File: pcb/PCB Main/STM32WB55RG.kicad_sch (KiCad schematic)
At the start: 26 parts, among them CN1 Conn_ARM_JTAG_SWD_10, SW1 SW_Push, U1 STM32WB55RGVx, Y1 32MHz, Y2 32.768kHz

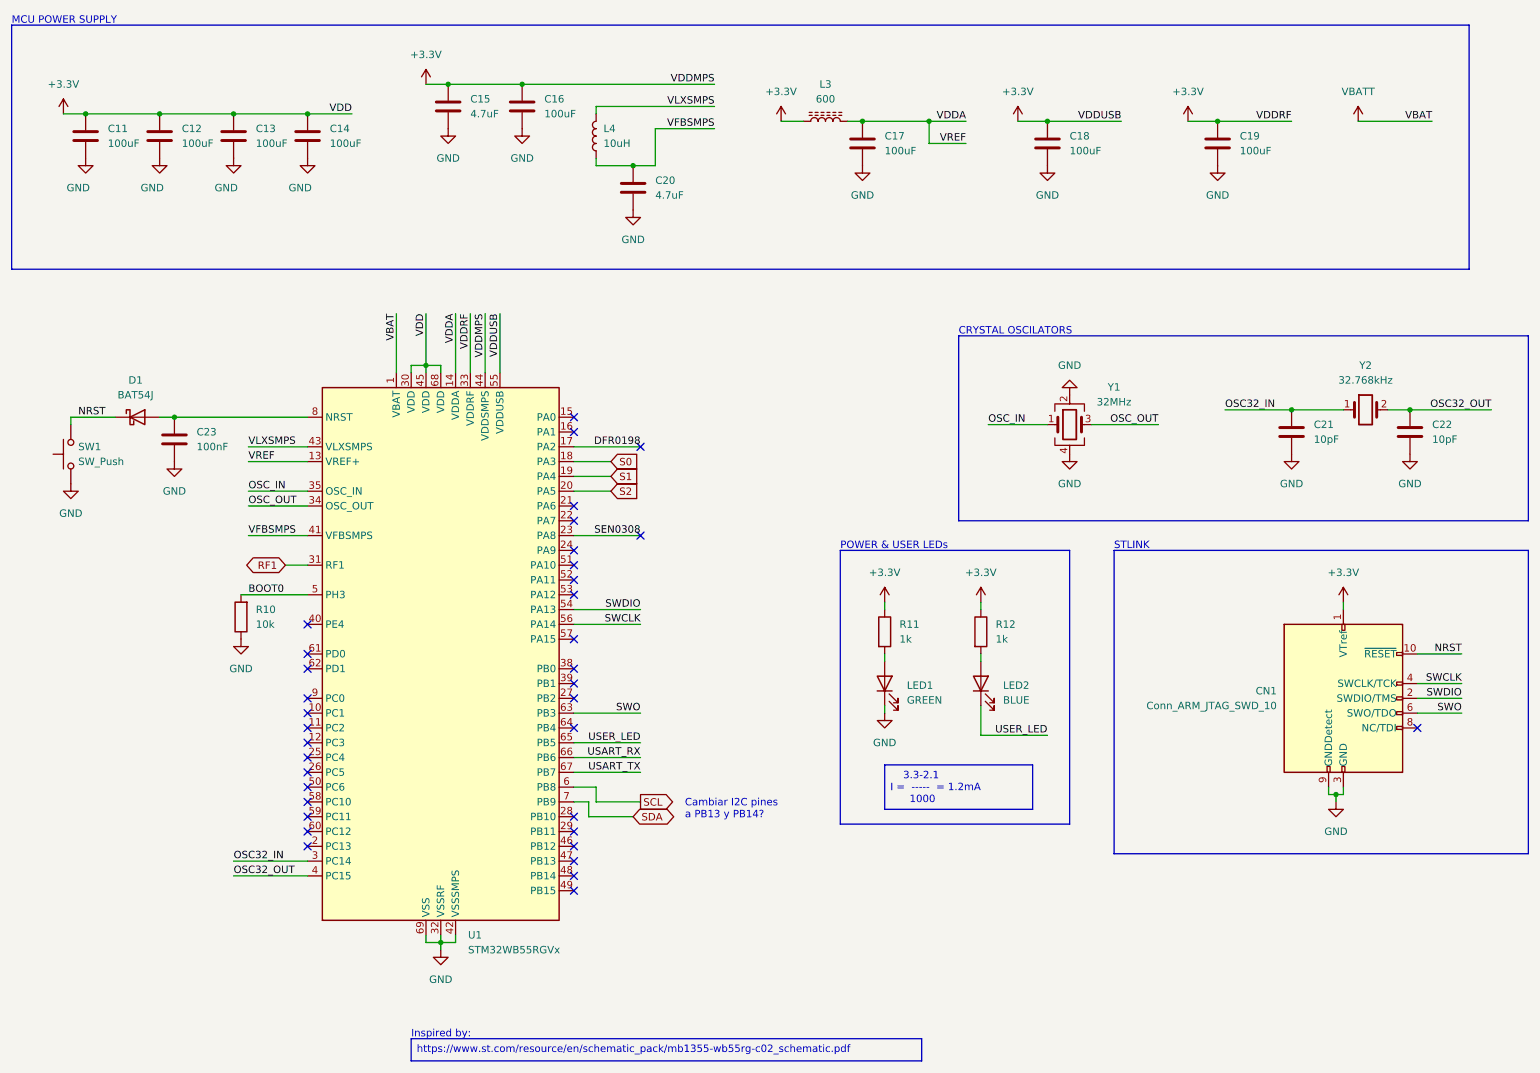
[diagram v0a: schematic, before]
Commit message: PCB casi lista
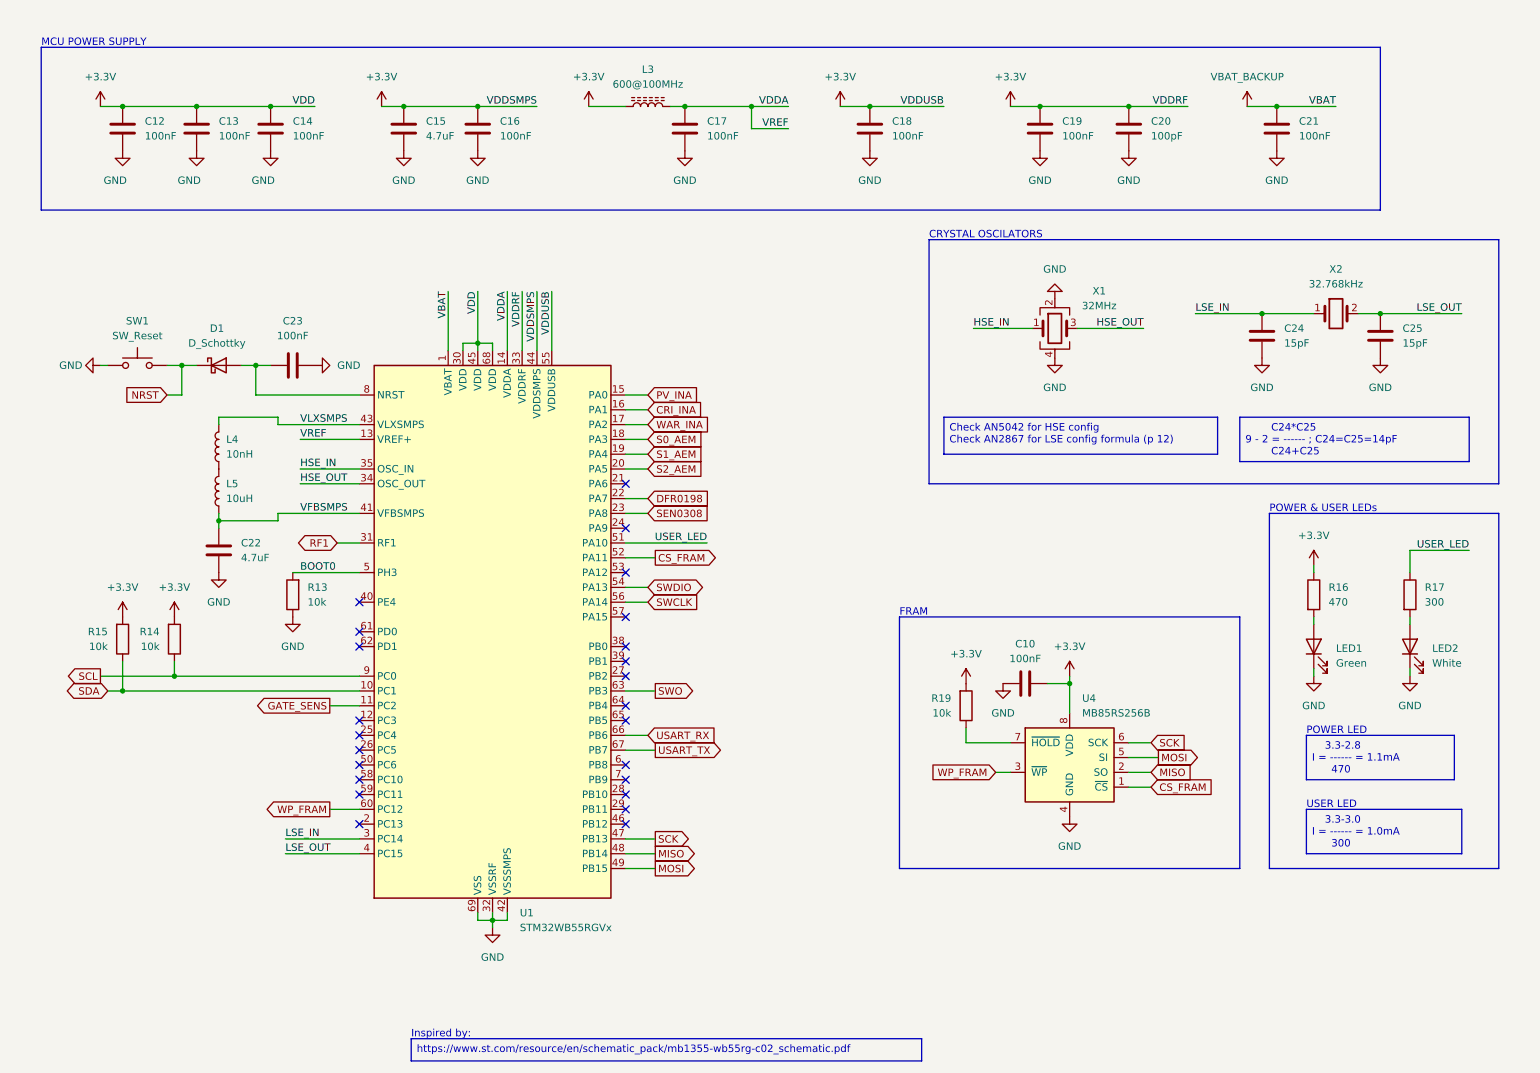
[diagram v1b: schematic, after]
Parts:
- removed C11: 100uF, symbol Device:C
- removed CN1: Conn_ARM_JTAG_SWD_10, Connector_PinHeader_1.27mm:PinHeader_2x05_P1.27mm_Vertical, symbol Connector:Conn_ARM_JTAG_SWD_10
- removed D1: BAT54J, Diode_SMD:D_SOD-323F, symbol Diode:BAT54J
- added C10, C21: 100nF, Capacitor_SMD:C_0402_1005Metric, symbol Device:C
- added C20: 100pF, Capacitor_SMD:C_0402_1005Metric, symbol Device:C
- added D1: D_Schottky, Diode_SMD:D_SOD-323, symbol Device:D_Schottky
- added L4: 10nH, Inductor_SMD:L_0402_1005Metric, symbol Device:L
- added R14, R15, R19: 10k, Resistor_SMD:R_0402_1005Metric, symbol Device:R
- added U4: MB85RS256B, Package_SO:SOIC-8_3.9x4.9mm_P1.27mm, symbol Memory_NVRAM:MB85RS256B
- C12, C13, C14, C16, C17, C18, C19: value 100uF -> 100nF; footprint (none) -> Capacitor_SMD:C_0402_1005Metric; Component (none) -> CL05B104KO5NNNC; Manufacturer (none) -> Samsung; Package (none) -> 0402; Supplier (none) -> JLCPCB; Supplier Part # (none) -> C1525; Supplier Part Type (none) -> Basic
- C15: footprint (none) -> Capacitor_SMD:C_0402_1005Metric; Component (none) -> CL05A475MP5NRNC; Manufacturer (none) -> Samsung; Package (none) -> 0402; Supplier (none) -> JLCPCB; Supplier Part # (none) -> C23733; Supplier Part Type (none) -> Basic
- C22: renamed from C20; footprint (none) -> Capacitor_SMD:C_0402_1005Metric; Component (none) -> CL05A475MP5NRNC; Manufacturer (none) -> Samsung; Package (none) -> 0402; Supplier (none) -> JLCPCB; Supplier Part # (none) -> C23733; Supplier Part Type (none) -> Basic
- C23: footprint (none) -> Capacitor_SMD:C_0402_1005Metric; Component (none) -> CL05B104KO5NNNC; Manufacturer (none) -> Samsung; Package (none) -> 0402; Supplier (none) -> JLCPCB; Supplier Part # (none) -> C1525; Supplier Part Type (none) -> Basic
- C24: renamed from C21; value 10pF -> 15pF; footprint (none) -> Capacitor_SMD:C_0402_1005Metric; Component (none) -> 0402CG150J500NT; Manufacturer (none) -> FH; Package (none) -> 0402; Supplier (none) -> JLCPCB; Supplier Part # (none) -> C1548; Supplier Part Type (none) -> Basic
- C25: renamed from C22; value 10pF -> 15pF; footprint (none) -> Capacitor_SMD:C_0402_1005Metric; Component (none) -> 0402CG150J500NT; Manufacturer (none) -> FH; Package (none) -> 0402; Supplier (none) -> JLCPCB; Supplier Part # (none) -> C1548; Supplier Part Type (none) -> Basic
- L3: value 600 -> 600@100MHz; Component FCM1608KF-601T02 -> GZ1608D601TF; Manufacturer TAI-TECH -> Sunlord; Package L_0603 -> 0603; Supplier Part # C127281 -> C1002; Supplier Part Type (none) -> Basic
- L5: renamed from L4; footprint (none) -> Inductor_SMD:L_0805_2012Metric; Component (none) -> SDFL2012S100KTF; Manufacturer (none) -> Sunlord; Package (none) -> 0805; Supplier (none) -> JLCPCB; Supplier Part # (none) -> C1046; Supplier Part Type (none) -> Basic
- LED1: value GREEN -> Green; footprint LED_SMD:LED_0603_1608Metric -> LED_SMD:LED_0805_2012Metric; Component APTD2012LCGCK -> KT-0805G; Manufacturer Kingbright -> Hubei KENTO Elec; Package LED_0805 -> 0805; Supplier Part # C5366381 -> C2297; Supplier Part Type (none) -> Basic
- LED2: value BLUE -> White; footprint LED_SMD:LED_0603_1608Metric -> LED_SMD:LED_0805_2012Metric; Component APTD2012LQBC/D -> KT-0805W; Manufacturer Kingbright -> Hubei KENTO Elec; Package LED_0805 -> 0805; Supplier Part # C5879058 -> C34499; Supplier Part Type (none) -> Basic
- R13: renamed from R10; footprint (none) -> Resistor_SMD:R_0402_1005Metric; Component (none) -> 0402WGF1002TCE; Manufacturer (none) -> UNI-ROYAL; Package (none) -> 0402; Supplier (none) -> JLCPCB; Supplier Part # (none) -> C25744; Supplier Part Type (none) -> Basic
- R16: renamed from R11; value 1k -> 470; footprint (none) -> Resistor_SMD:R_0402_1005Metric; Component (none) -> 0603WAF4700T5E; Manufacturer (none) -> UNI-ROYAL; Package (none) -> 0603; Supplier (none) -> JLCPCB; Supplier Part # (none) -> C23179; Supplier Part Type (none) -> Basic
- R17: renamed from R12; value 1k -> 300; footprint (none) -> Resistor_SMD:R_0402_1005Metric; Component (none) -> 0603WAF3000T5E; Manufacturer (none) -> UNI-ROYAL; Package (none) -> 0603; Supplier (none) -> JLCPCB; Supplier Part # (none) -> C23025; Supplier Part Type (none) -> Basic
- SW1: value SW_Push -> SW_Reset; Component 4*4*1.7 Surface Mount -> TS-1187A-B-A-B; Manufacturer BOOMELE (Boom Precision Elec) -> XKB Connection; Package SMD-4P 5.2x5.2mm -> SMD-4P 5.1x5.1mm; Supplier Part # C10852 -> C318884; Supplier Part Type (none) -> Basic
- U1: Manufacturer STMicroelectronics -> STMicroelectronics; Supplier Part Type (none) -> Extended
- X1: renamed from Y1; Component NX2016SA-32M-EXS00A-CS06465 -> NX2016SA-32M-EXS00A-CS06465; Supplier Part Type (none) -> Extended
- X2: renamed from Y2; Supplier Part Type (none) -> Extended
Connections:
- net +3.3V: now also C10.1, C20.2, R14.2, R15.2, R19.2, U4.8 (VDD); no longer R17.1
- net DFR0198: now also U1.22 (PA7); no longer U1.17 (PA2)
- net GND: now also LED2.1 (K), C10.2, C20.1, C21.1, U4.4 (GND)
- net NRST: now also D1.1 (K)
- net SCL: now also U1.9 (PC0), R14.1; no longer U1.6 (PB8)
- net SDA: now also U1.10 (PC1), R15.1; no longer U1.7 (PB9)
- net USER_LED: now also R17.1, U1.51 (PA10); no longer LED2.1 (K), U1.65 (PB5)
- net VLXSMPS: now also L4.2; no longer L5.2
- net at C23.2, U1.8 (NRST): now also D1.2 (A)
- net GATE_SENS: now reaches U1.11 (PC2)
- net PV_INA: now reaches U1.15 (PA0)
- net CRI_INA: now reaches U1.16 (PA1)
- net SCK: now reaches U1.47 (PB13)
- net SCK: now also U4.6 (SCK)
- net MISO: now reaches U1.48 (PB14)
- net MISO: now also U4.2 (SO)
- net MOSI: now reaches U1.49 (PB15)
- net MOSI: now also U4.5 (SI)
- net CS_FRAM: now reaches U1.52 (PA11)
- net CS_FRAM: now also U4.1 (~{CS})
- net WP_FRAM: now reaches U1.60 (PC12)
- net WP_FRAM: now also U4.3 (~{WP})
- net OSC32_IN renamed LSE_IN
- net OSC32_OUT renamed LSE_OUT
- net OSC_IN renamed HSE_IN
- net OSC_OUT renamed HSE_OUT
- net S0 renamed S0_AEM
- net S1 renamed S1_AEM
- net S2 renamed S2_AEM
- net VBATT renamed VBAT_BACKUP
- net VBAT_BACKUP: now also C21.2
- new net: L4.1, L5.2
- new net: R19.1, U4.7 (~{HOLD})
- new net WAR_INA: U1.17 (PA2)
- no-connect marks 36 -> 24
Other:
- note added: "FRAM"
- note added: "POWER LED"
- note added: "USER LED"
- note removed: "Cambiar I2C pines a PB13 y PB14?"
- note removed: "STLINK"
- moved on the sheet: C12, C13, C14, C15, C16, C17, C18, C19, C22, C24, C25, L3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
